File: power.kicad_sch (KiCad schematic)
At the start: 12 parts, among them SW3 SW_SPDT, U2 TP4054, U4 XC6206PxxxMR

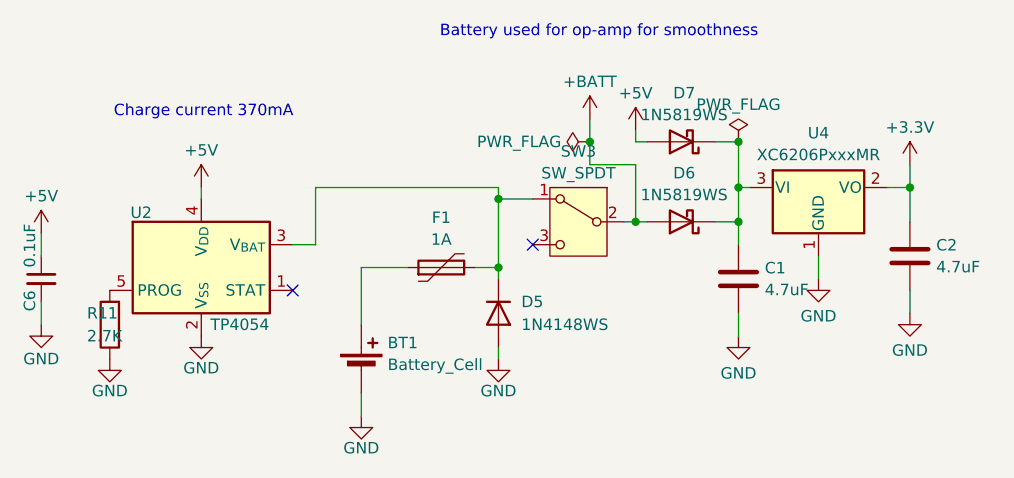
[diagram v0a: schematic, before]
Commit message: stm32g0
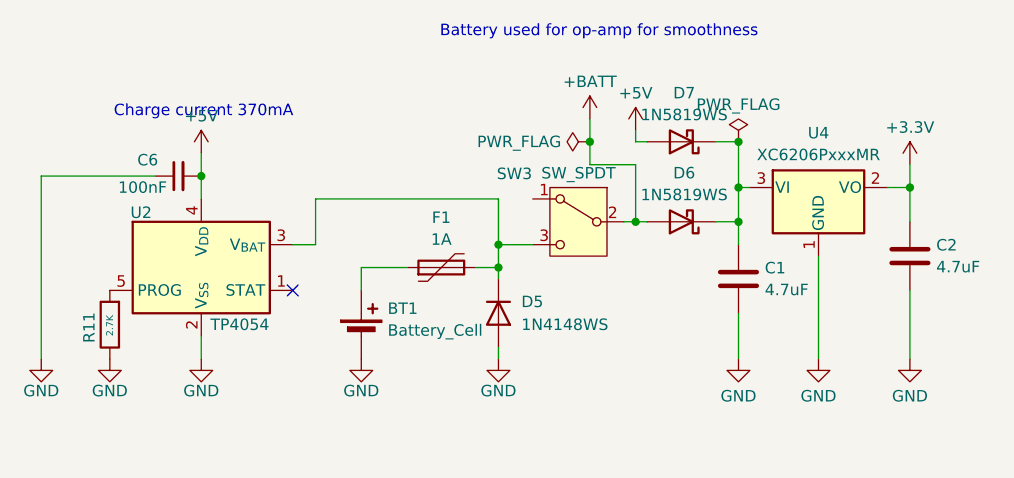
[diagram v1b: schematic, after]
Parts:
- C6: value 0.1uF -> 100nF
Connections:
- net +5V: now also C6.2; no longer C6.1
- net GND: now also C6.1; no longer C6.2
- net at D5.1 (K), F1.2, U2.3 (V_{BAT}): now also SW3.3 (C); no longer SW3.1 (A)
- no-connect marks 2 -> 1
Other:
- moved on the sheet: BT1, C6
